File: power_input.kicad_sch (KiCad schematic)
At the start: 0 parts

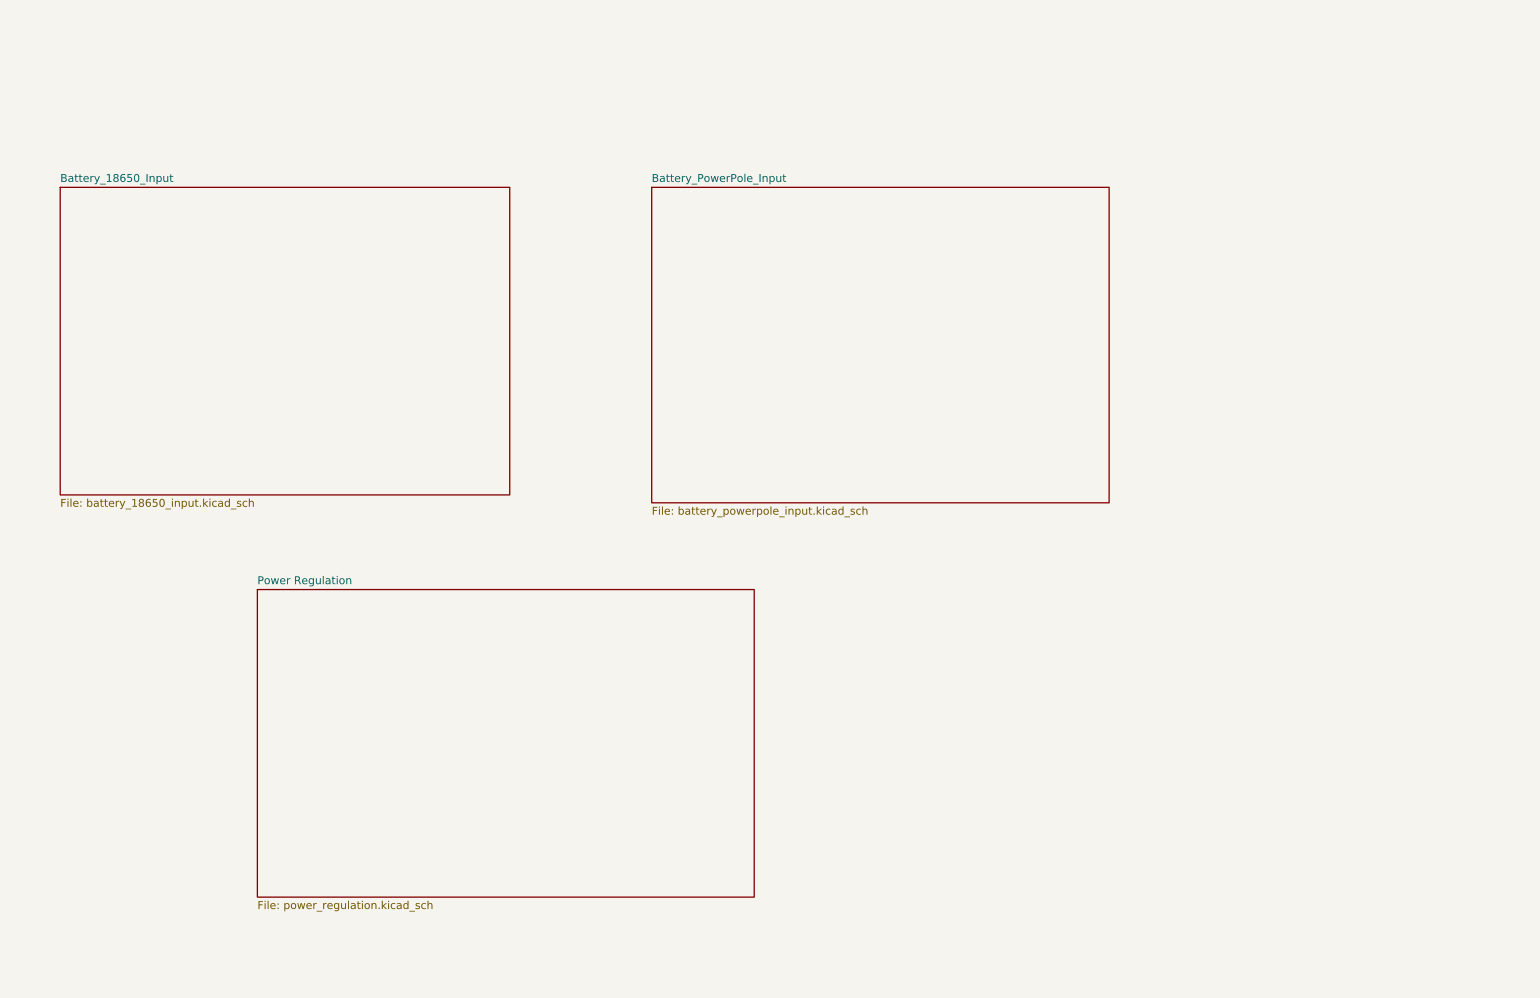
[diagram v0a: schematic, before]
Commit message: hierarchy work
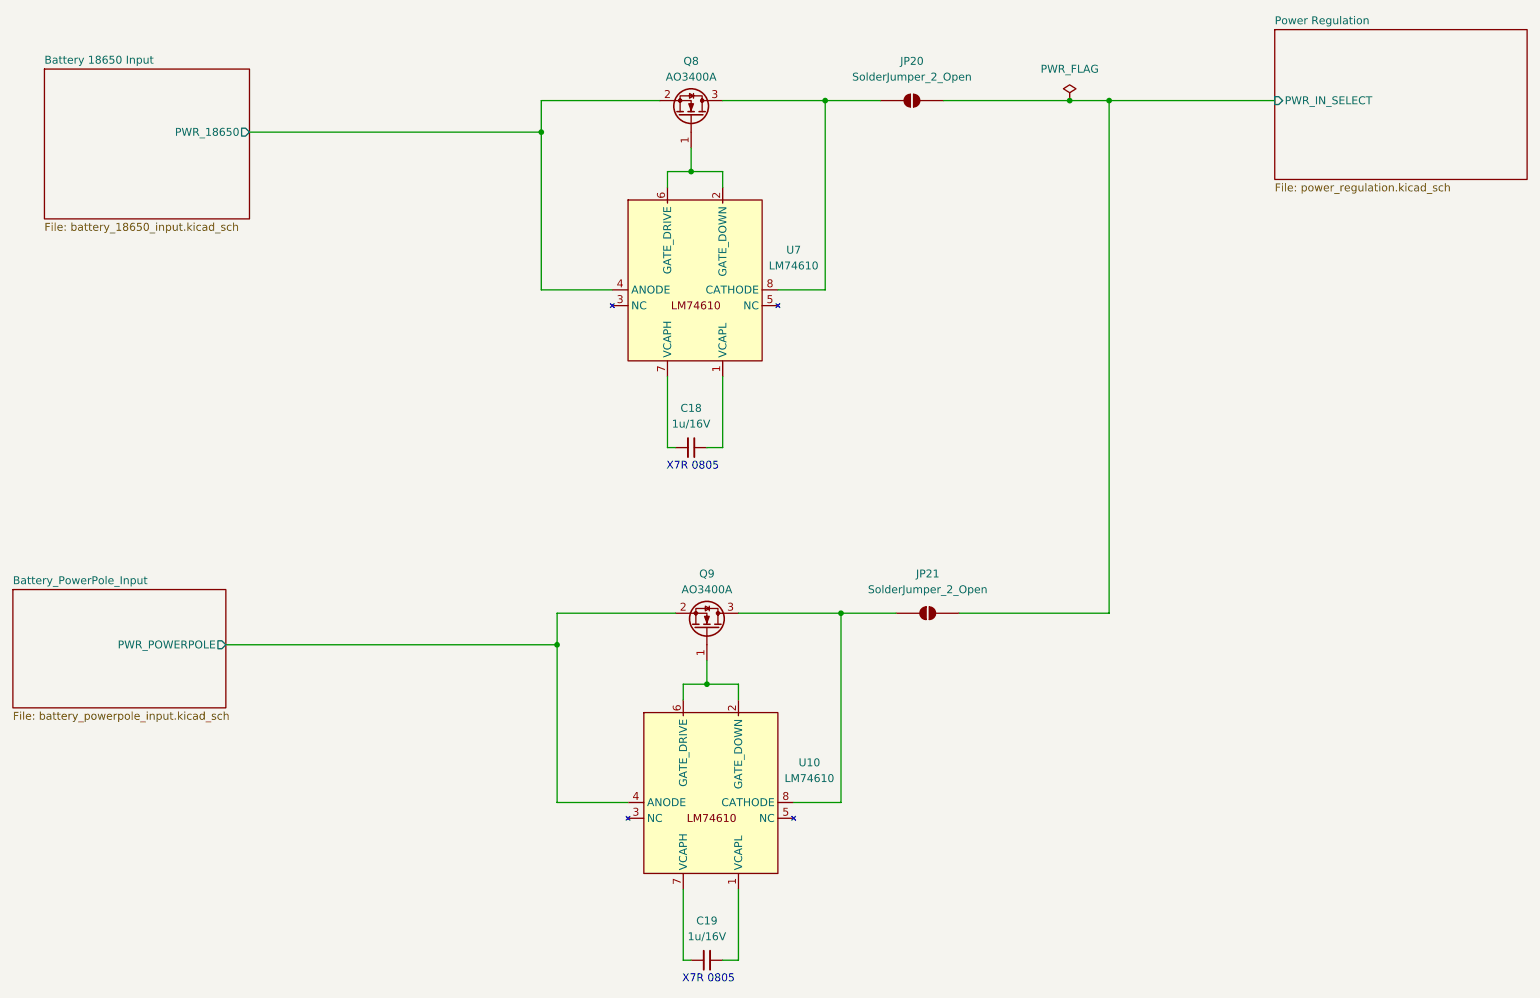
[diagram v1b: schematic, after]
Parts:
- added C18, C19: 1u/16V, Capacitor_SMD:C_0805_2012Metric, symbol Device:C_Small
- added JP20, JP21: SolderJumper_2_Open, Jumper:SolderJumper-2_P1.3mm_Open_TrianglePad1.0x1.5mm, symbol Jumper:SolderJumper_2_Open
- added Q8, Q9: AO3400A, Package_TO_SOT_SMD:SOT-23, symbol Transistor_FET:AO3400A
- added U10, U7: LM74610, Package_SO:VSSOP-8_3x3mm_P0.65mm, symbol kicad_gx_library:LM74610
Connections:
- new net: C18.2, U7.1 (VCAPL)
- new net: Q8.1 (G), U7.2 (GATE_DOWN), U7.6 (GATE_DRIVE)
- new net: C18.1, U7.7 (VCAPH)
- new net: JP20.1 (A), Q8.3 (D), U7.8 (CATHODE)
- new net: C19.1, U10.7 (VCAPH)
- new net: C19.2, U10.1 (VCAPL)
- new net: Q9.1 (G), U10.2 (GATE_DOWN), U10.6 (GATE_DRIVE)
- new net: JP21.1 (A), Q9.3 (D), U10.8 (CATHODE)
- new net Battery 18650 Input/PWR_18650: Q8.2 (S), U7.4 (ANODE)
- new net Battery_PowerPole_Input/PWR_POWERPOLE: Q9.2 (S), U10.4 (ANODE)
- new net Power Regulation/PWR_IN_SELECT: JP20.2 (B), JP21.2 (B)
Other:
- removed sheet Battery_18650_Input
- added sheet Battery 18650 Input (battery_18650_input.kicad_sch)
- sheet Battery_PowerPole_Input ports: added PWR_POWERPOLE; removed none
- sheet Power Regulation ports: added PWR_IN_SELECT; removed none
- note added: "X7R 0805"
